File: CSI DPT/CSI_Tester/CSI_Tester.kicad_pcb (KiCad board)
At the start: 4 copper layers, 100 x 80 mm, 49 parts, among them J2 Conn_02x08_Odd_Even, J3 SSW-102-01-G-D, Q3 DMP3099L, U1 UCC23513QDWYRQ1, U2 MGJ2D121802SC, U4 LDK130-12_SOT23_SOT353, U5 NC7SZ125M5X, U7 ADM4168EBRUZ, U8 MGJ2D121802SC, U9 LT1086-ADJ

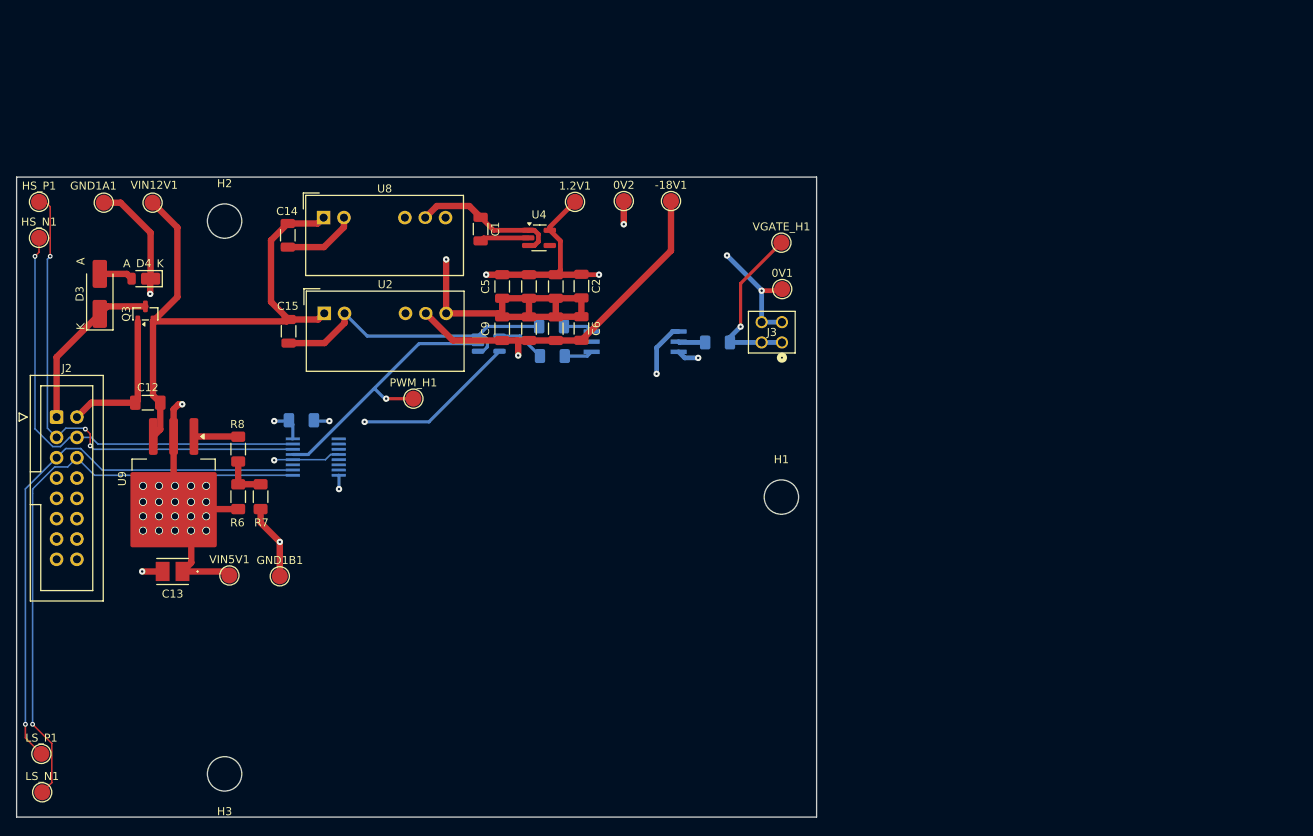
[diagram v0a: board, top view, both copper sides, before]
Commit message: CSI Tester V1 Completed
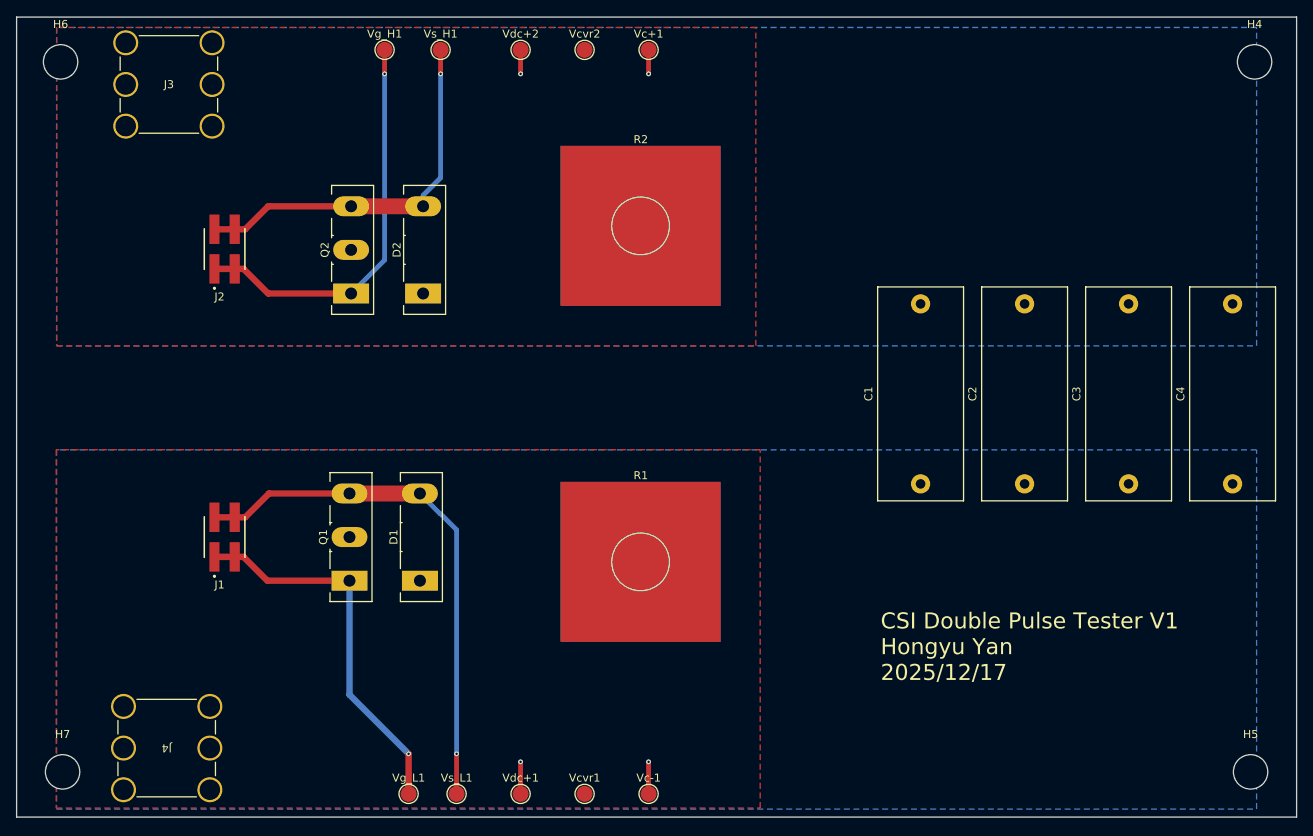
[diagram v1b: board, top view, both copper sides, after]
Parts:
- removed -18V1, 0V1, 0V2, 1.2V1, GND1A1, GND1B1, PWM_H1, VGATE_H1, VIN12V1, VIN5V1: TestPoint, TestPoint:TestPoint_Pad_D2.0mm
- removed C11: 0.1u, Capacitor_SMD:C_1206_3216Metric_Pad1.33x1.80mm_HandSolder
- removed C12: 10u, Capacitor_SMD:C_1206_3216Metric_Pad1.33x1.80mm_HandSolder
- removed C13: 10u, Gate_Driver:TAJB_AVX-M
- removed C14, C15: 10u, Capacitor_SMD:C_1206_3216Metric
- removed C5, C6, C7, C8, C9: 1u, Capacitor_SMD:C_1206_3216Metric
- removed D3: Z1SMAxxx, Diode_SMD:D_SMA_Handsoldering
- removed D4: D_Schottky, Diode_SMD:D_PowerDI-123
- removed H1, H2, H3: MountingHole, MountingHole:MountingHole_4.3mm_M4_DIN965
- removed HS_N1: HS_N, TestPoint:TestPoint_Pad_D2.0mm
- removed HS_P1: HS_P, TestPoint:TestPoint_Pad_D2.0mm
- removed LS_N1: LS_N, TestPoint:TestPoint_Pad_D2.0mm
- removed LS_P1: LS_P, TestPoint:TestPoint_Pad_D2.0mm
- removed Q3: DMP3099L, Package_TO_SOT_SMD:SOT-23
- removed R3, R4: 145, Resistor_SMD:R_1206_3216Metric_Pad1.30x1.75mm_HandSolder
- removed R6: 121, Resistor_SMD:R_1206_3216Metric_Pad1.30x1.75mm_HandSolder
- removed R7: 365, Resistor_SMD:R_1206_3216Metric_Pad1.30x1.75mm_HandSolder
- removed R8: 0, Resistor_SMD:R_1206_3216Metric_Pad1.30x1.75mm_HandSolder
- removed U1: UCC23513QDWYRQ1, Gate_Driver:SOIC06_SO-6_7P5X4P68_TEX-M
- removed U2, U8: MGJ2D121802SC, Converter_DCDC:Converter_DCDC_Murata_MGJ2DxxxxxxSC_THT
- removed U4: LDK130-12_SOT23_SOT353, Package_TO_SOT_SMD:SOT-23-5_HandSoldering
- removed U5: NC7SZ125M5X, Package_TO_SOT_SMD:SOT-23-5_HandSoldering
- removed U7: ADM4168EBRUZ, Gate_Driver:RU_16_ADI-M
- removed U9: LT1086-ADJ, Package_TO_SOT_SMD:TO-263-3_TabPin2
- added D1: UJ3N065025K3S, Package_TO_SOT_THT:TO-247-2_Vertical, F.Cu at (116.4, 112.3)
- added D2: UJ3N065025K3S, Package_TO_SOT_THT:TO-247-2_Vertical, F.Cu at (116.8, 76.5)
- added H4: MountingHole, MountingHole:MountingHole_4.3mm_M4_DIN965, F.Cu at (220.8, 47.5)
- added H5: MountingHole, MountingHole:MountingHole_4.3mm_M4_DIN965, F.Cu at (220.2, 136.2)
- added H6: MountingHole, MountingHole:MountingHole_4.3mm_M4_DIN965, F.Cu at (71.5, 47.5)
- added H7: MountingHole, MountingHole:MountingHole_4.3mm_M4_DIN965, F.Cu at (71.8, 136.2)
- added J1: TSM-102-01-SM-DV, VSI_DPT:SAMTEC_TSM-102-01-SM-DV, F.Cu at (92.0, 106.9)
- added J4: 8196, CSI_DPT:CONN_8196_KEY, F.Cu at (90.2, 138.5)
- added Q1: UJ3N065025K3S, Package_TO_SOT_THT:TO-247-3_Vertical, F.Cu at (107.6, 112.3)
- added Q2: UJ3N065025K3S, Package_TO_SOT_THT:TO-247-3_Vertical, F.Cu at (107.8, 76.5)
- added R2: CVR, Resistor_THT:CVR_SSDN005, F.Cu at (144.0, 68.0)
- added Vc+1: Vc+, TestPoint:TestPoint_Pad_D2.0mm, F.Cu at (145.0, 46.0)
- added Vc-1: TP1, TestPoint:TestPoint_Pad_D2.0mm, F.Cu at (145.0, 139.0)
- added Vcvr1: ~, TestPoint:TestPoint_Pad_D2.0mm, F.Cu at (137.0, 139.0)
- added Vcvr2: ~, TestPoint:TestPoint_Pad_D2.0mm, F.Cu at (137.0, 46.0)
- added Vdc+1: ~, TestPoint:TestPoint_Pad_D2.0mm, F.Cu at (129.0, 139.0)
- added Vdc+2: ~, TestPoint:TestPoint_Pad_D2.0mm, F.Cu at (129.0, 46.0)
- added Vg_H1: Vc+, TestPoint:TestPoint_Pad_D2.0mm, F.Cu at (112.0, 46.0)
- added Vg_L1: Vg_L, TestPoint:TestPoint_Pad_D2.0mm, F.Cu at (115.0, 139.0)
- added Vs_H1: Vc+, TestPoint:TestPoint_Pad_D2.0mm, F.Cu at (119.0, 46.0)
- added Vs_L1: Vc+, TestPoint:TestPoint_Pad_D2.0mm, F.Cu at (121.0, 139.0)
- C1, C2, C3, C4: value 1u -> 0.15u; footprint Capacitor_SMD:C_1206_3216Metric -> Capacitor_THT:C_Rect_L26.5mm_W10.5mm_P22.50mm_MKS4
- J2: value Conn_02x08_Odd_Even -> TSM-102-01-SM-DV; footprint Connector_IDC:IDC-Header_2x08_P2.54mm_Vertical -> VSI_DPT:SAMTEC_TSM-102-01-SM-DV
- J3: value SSW-102-01-G-D -> 8196; footprint Gate_Driver:CON4_2X2_TU_SSQ -> CSI_DPT:CONN_8196_KEY
- R1: value Ron 2 ohm -> CVR; footprint Resistor_SMD:R_1206_3216Metric_Pad1.30x1.75mm_HandSolder -> Resistor_THT:CVR_SSDN005; moved to F.Cu
- moved C4 91.3 mm to (218.0, 100.2), turned to 90 degrees
- moved J3 88.5 mm to (79.6, 45.1)
- moved C3 75.7 mm to (205.0, 100.2), turned to 90 degrees
- moved C1 63.6 mm to (179.0, 100.2), turned to 90 degrees
- moved C2 60.7 mm to (192.0, 100.2), turned to 90 degrees
- moved J2 29.7 mm to (92.0, 70.9), turned to 180 degrees
- moved R1 29.1 mm to (144.0, 110.0), turned to 0 degrees
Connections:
- net /Gate_Driver/0V_H renamed /Tester_Board/Vc+
- C1 pad 1: Net-(U4-EN) -> /Tester_Board/Vc-
- C2 pad 1: /Gate_Driver/1.2V_H -> /Tester_Board/Vc-
- C3 pad 1: /Gate_Driver/1.2V_H -> /Tester_Board/Vc-
- C4 pad 1: /Gate_Driver/1.2V_H -> /Tester_Board/Vc-
- J3 pad 1: /Gate_Driver/VGATE_H -> /Tester_Board/Vdc+
- J3 pad 2: /Gate_Driver/0V -> /Tester_Board/Vdc+
- J3 pad 3: /Gate_Driver/VGATE_H -> /Tester_Board/Vdc+
- J3 pad 4: /Gate_Driver/0V -> /Tester_Board/Vdc+
- R1 pad 1: /Gate_Driver/VGATE_H -> /Tester_Board/Vcvr1
- R1 pad 2: Net-(U1-VOUT) -> /Tester_Board/Vc-
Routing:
- net GND1: track 106.3 -> 0.00 mm, vias 5 -> 0
- net /Gate_Driver/LS_N: track 74.5 -> 0.00 mm, vias 1 -> 0
- net /Gate_Driver/VIN12V: track 72.9 -> 0.00 mm
- net /Gate_Driver/LS_P: track 70.6 -> 0.00 mm, vias 1 -> 0
- net /Tester_Board/Vs_L: track 0.00 -> 66.4 mm, vias 0 -> 1
- net /Gate_Driver/HS_P: track 63.1 -> 0.00 mm, vias 3 -> 0
- net /Gate_Driver/VIN5V: track 61.4 -> 0.00 mm, vias 24 -> 0
- net /Gate_Driver/HS_N: track 58.0 -> 0.00 mm, vias 1 -> 0
- net /Gate_Driver/-18V_H: track 51.7 -> 0.00 mm, vias 2 -> 0
- net /Tester_Board/Vg_H: track 0.00 -> 50.5 mm, vias 0 -> 1
- net /Tester_Board/Vc+: track 52.1 -> 3.00 mm, vias 0 -> 1
- net /Tester_Board/Vg_L: track 0.00 -> 47.8 mm, vias 0 -> 1
- net /Tester_Board/Vs_H: track 0.00 -> 47.7 mm, vias 0 -> 1
- net /Gate_Driver/PWM_H: track 34.3 -> 0.00 mm, vias 1 -> 0
- net /Gate_Driver/1.2V_H: track 28.1 -> 0.00 mm, vias 3 -> 0
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- added copper zone on B.Cu, net /Tester_Board/Vc+
- added copper zone on B.Cu, net /Tester_Board/Vc-
- added copper zone on F.Cu, net /Tester_Board/Vcvr1
- added copper zone on F.Cu, net /Tester_Board/Vcvr2
- added copper zone on In1.Cu, net /Tester_Board/Vdc+
- removed copper zone on In1.Cu, net /Gate_Driver/-18V_H
- removed copper zone on In1.Cu, net /Gate_Driver/0V
- removed copper zone on In1.Cu, net /Gate_Driver/1.2V_H
- removed copper zone on In2.Cu, net /Gate_Driver/VIN5V
- removed copper zone on In1.Cu, net GND1
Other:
- board size 100 x 80 mm -> 160 x 100 mm
- board text added: "CSI Double Pulse Tester V1 Hongyu Yan 2025/12/17"
- board text removed: "A"
- board text removed: "K"
